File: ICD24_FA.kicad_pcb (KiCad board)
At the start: 2 copper layers, 146.5 x 123.5 mm, 116 parts, among them J81 Conn_01x02, Q1 2N3904, Q10 2N3904, Q11 2N3904, Q12 2N3904, Q13 2N3904, Q14 2N3904, Q15 2N3904, Q16 2N3904, Q17 2N3904, Q18 2N3904, Q19 2N3904, Q2 2N3904, Q3 2N3904, Q4 2N3904, Q5 2N3904, Q574 2N3904, Q575 2N3904, Q576 2N3904, Q577 2N3904, Q578 2N3904, Q579 2N3904, Q580 2N3904, Q581 2N3904, Q582 2N3904, Q583 2N3904, Q584 2N3904, Q585 2N3904, Q586 2N3904, Q587 2N3904, Q588 2N3904, Q589 2N3904, Q590 2N3904, Q591 2N3904, Q592 2N3904, Q6 2N3904, Q7 2N3904, Q8 2N3904, Q9 2N3904, SW81 SW_SPDT, SW82 SW_SPDT, SW83 SW_SPDT, SW84 SW_SPDT, SW97 SW_SPDT

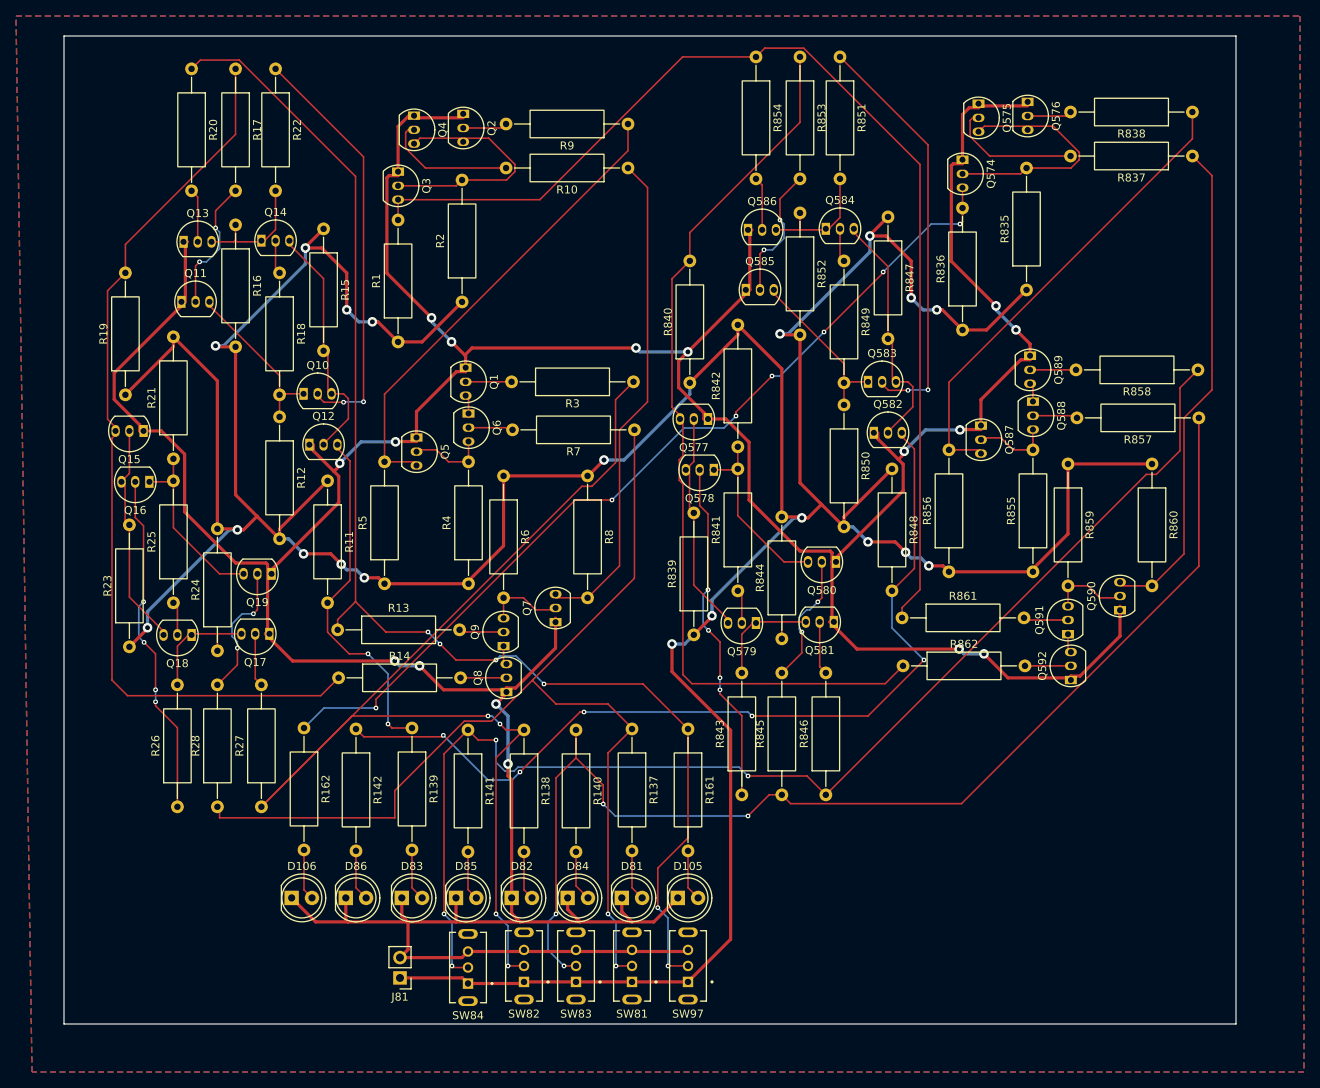
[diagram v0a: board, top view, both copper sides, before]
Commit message: FA 1-Bit PCB ok
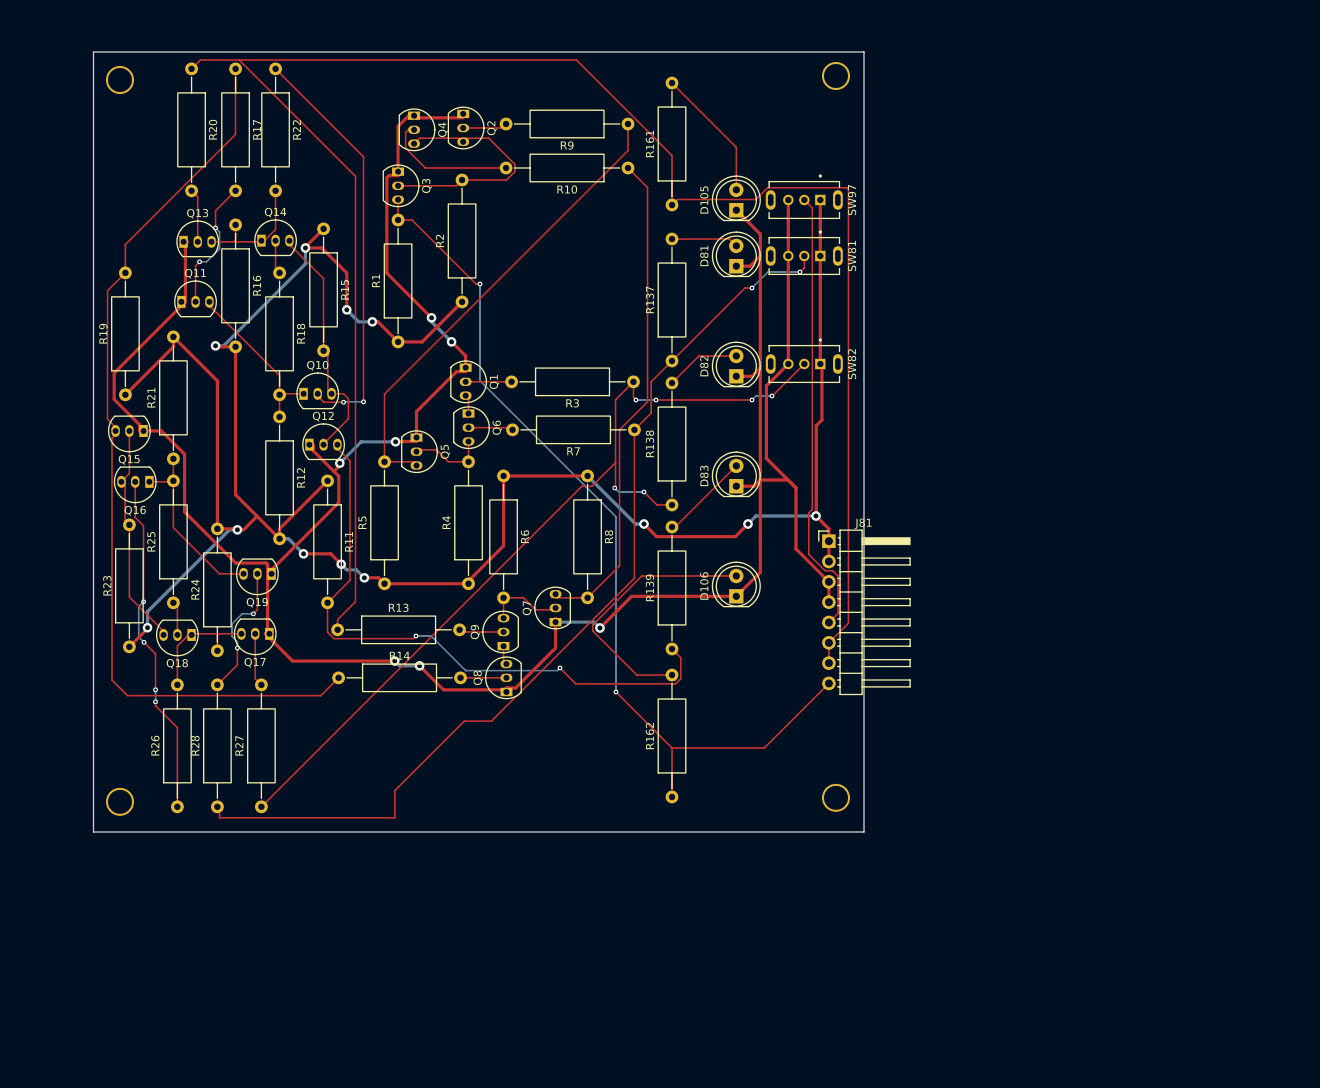
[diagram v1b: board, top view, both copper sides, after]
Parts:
- removed D84, D85, D86: LED, LED_THT:LED_D5.0mm
- removed Q574, Q575, Q576, Q577, Q578, Q579, Q580, Q581, Q582, Q583, Q584, Q585, Q586, Q587, Q588, Q589, Q590, Q591, Q592: 2N3904, MyLibrary:TO-92_Inline
- removed R140, R141, R142, R836, R840, R848, R856, R860: 47k, Resistor_THT:R_Axial_DIN0309_L9.0mm_D3.2mm_P15.24mm_Horizontal
- removed R835, R837, R838, R839, R841, R842, R843, R844, R845, R846, R847, R849, R850, R851, R852, R853, R854, R855, R857, R858, R859, R861, R862: 220k, Resistor_THT:R_Axial_DIN0309_L9.0mm_D3.2mm_P15.24mm_Horizontal
- removed SW83, SW84: SW_SPDT, MyLibrary:SW_SS12D07VG4
- added R20: 220k, MyLibrary:MyPAD, F.Cu at (101.0, 118.0)
- added R20: 220k, MyLibrary:MyPAD, F.Cu at (190.5, 207.7)
- added R20: 220k, MyLibrary:MyPAD, F.Cu at (190.5, 117.5)
- added R20: 220k, MyLibrary:MyPAD, F.Cu at (101.0, 208.2)
- J81: value Conn_01x02 -> Conn_01x08; footprint Connector_PinHeader_2.54mm:PinHeader_1x02_P2.54mm_Vertical -> Connector_PinHeader_2.54mm:PinHeader_1x08_P2.54mm_Horizontal
- moved SW97 96.8 mm to (186.5, 133.0), turned to 180 degrees
- moved SW81 91.3 mm to (186.5, 140.0), turned to 180 degrees
- moved D105 86.3 mm to (178.0, 134.3), turned to 90 degrees
- moved SW82 83.0 mm to (186.5, 153.5), turned to 180 degrees
- moved D81 80.3 mm to (178.0, 141.3), turned to 90 degrees
- moved J81 76.5 mm to (189.6, 175.7), turned to 0 degrees
- moved D82 71.0 mm to (178.0, 155.0), turned to 90 degrees
- moved D106 67.2 mm to (178.0, 182.5), turned to 90 degrees
- moved D83 66.3 mm to (178.0, 168.8), turned to 90 degrees
- moved R161 65.5 mm to (170.0, 133.6), turned to 90 degrees
- moved R162 46.8 mm to (170.0, 207.6), turned to 90 degrees
- moved R137 46.3 mm to (170.0, 153.1), turned to 90 degrees
- moved R139 34.0 mm to (170.0, 189.1), turned to 90 degrees
- moved R138 33.7 mm to (170.0, 171.1), turned to 90 degrees
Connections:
- net /fa2_bit/fa1/and_gate/IN_B renamed /fa1_bit/fa1/and_gate/IN_B
- net /fa2_bit/fa1/and_gate/OUT renamed /fa1_bit/fa1/and_gate/OUT
- net /fa2_bit/fa1/and_gate1/OUT renamed /fa1_bit/fa1/and_gate1/OUT
- J81 pad 2: 0 -> VDD
- Q3 pad 3: /fa2_bit/fa1/CARRY_OUT -> OUT_COUT
- R1 pad 2: /fa2_bit/fa1/CARRY_OUT -> OUT_COUT
- SW97 pad 2: CIN -> CIN_Port
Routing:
- net VDD: track 511.1 -> 281.9 mm, vias 20 -> 12
- net 0: track 567.2 -> 345.7 mm, vias 16 -> 7
- net IN_B1: track 156.5 -> 0.00 mm, vias 4 -> 0
- net IN_A1: track 147.9 -> 0.00 mm, vias 4 -> 0
- net /fa2_bit/fa1/CARRY_OUT: track 139.7 -> 0.00 mm
- net /fa2_bit/fa2/and_gate/IN_B: track 113.8 -> 0.00 mm
- net OUT_SUM1: track 112.5 -> 0.00 mm, vias 5 -> 0
- net CIN: track 167.4 -> 232.7 mm, vias 6 -> 0
- net /fa2_bit/fa2/and_gate/OUT: track 61.8 -> 0.00 mm
- net /fa2_bit/fa2/and_gate1/OUT: track 58.8 -> 0.00 mm
- net CIN_Port: track 0.00 -> 56.0 mm
- net Net-(Q583-B): track 52.5 -> 0.00 mm, vias 2 -> 0
- net Net-(Q578-B): track 43.3 -> 0.00 mm, vias 4 -> 0
- net IN_B0: track 144.9 -> 109.7 mm, vias 4 -> 6
- net OUT_SUM0: track 44.6 -> 77.3 mm
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- removed copper zone on B.Cu, net 0
- removed copper zone on F.Cu, net 0
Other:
- board size 146.5 x 123.5 mm -> 96.3 x 97.5 mm
